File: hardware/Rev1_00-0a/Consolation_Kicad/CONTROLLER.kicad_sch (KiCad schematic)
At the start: 50 parts, among them J11 5051101092, J13 5051101092, J14 SFV5R-2STBE1HLF, J15 SFV5R-2STBE1HLF, U2 RP2350A, U7 ECS-2016MVQ-120-BP-TR, U8 GD25Q32CWIGR

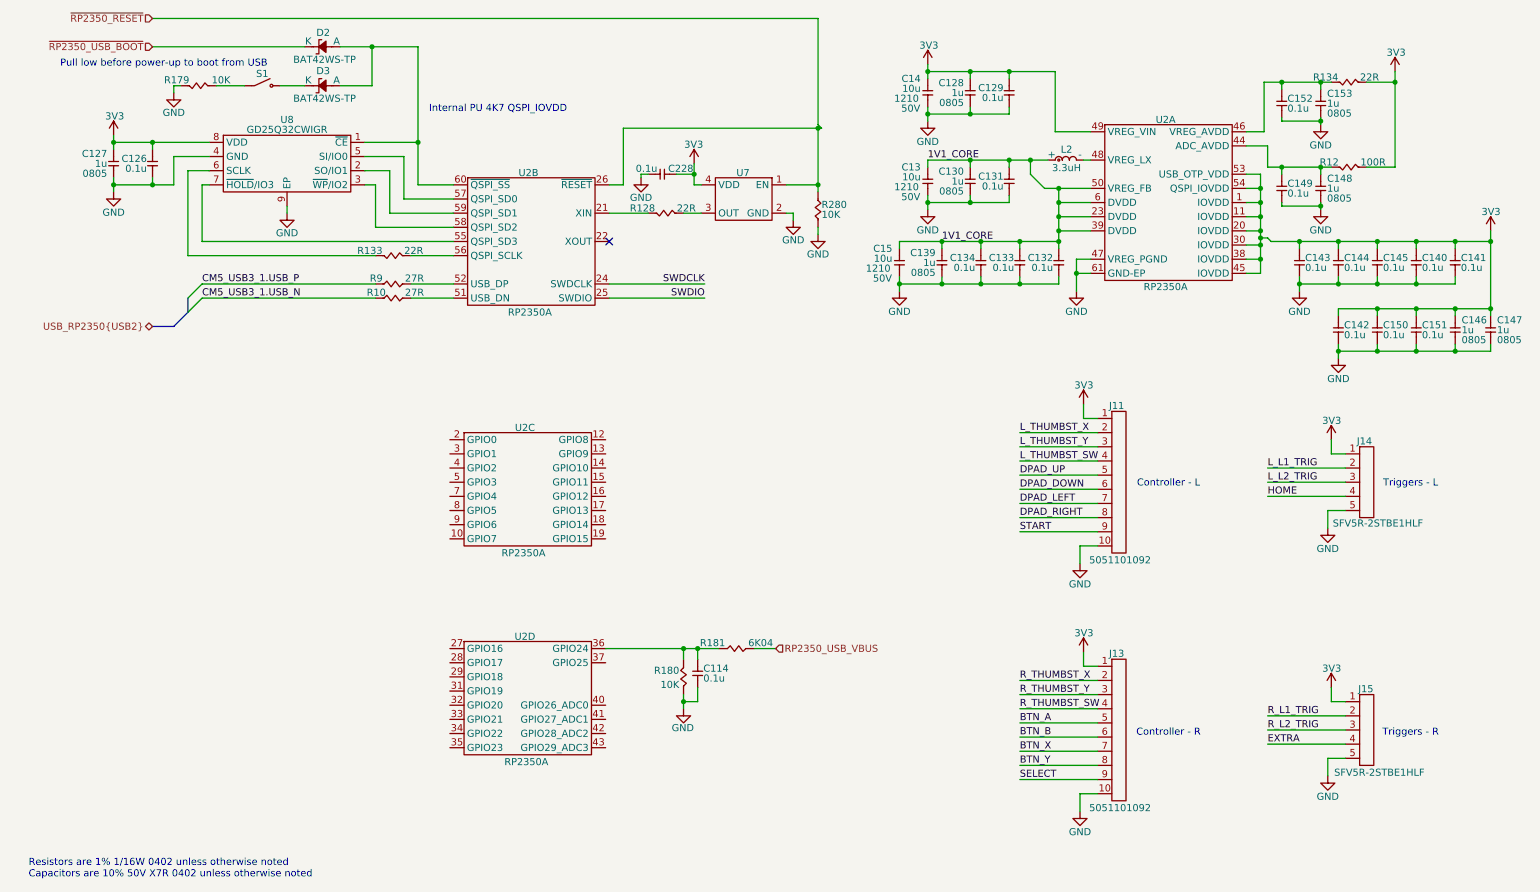
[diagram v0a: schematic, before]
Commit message: Update PinMux & Schematics
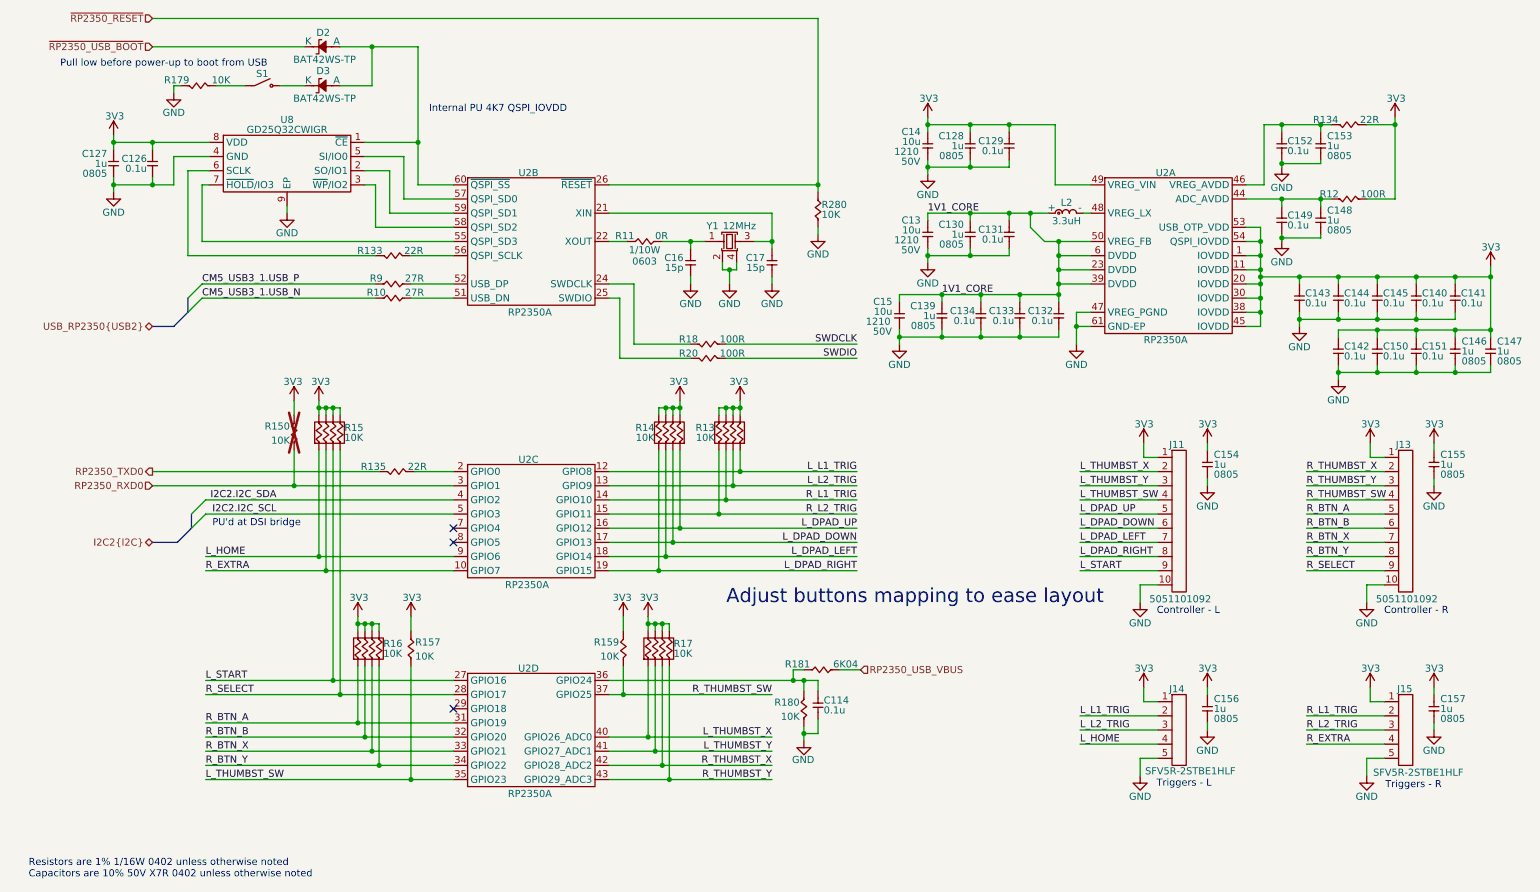
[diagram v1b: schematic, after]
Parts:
- removed C228: 0.1u, footprint:CAP_NONPOL_0402, symbol KicadCompDb:Capacitors/CAP_CER_SMT_00001
- removed R128: 22R, footprint:RES_0402, symbol KicadCompDb:Resistors/RES_SMT_00015
- removed U7: ECS-2016MVQ-120-BP-TR, footprint:4-SMD_2mmx1_6mm, symbol KicadCompDb:Oscillator/OSC_00003
- added C154, C155, C156, C157: 1u, footprint:CAP_NONPOL_0805, symbol KicadCompDb:Capacitors/CAP_CER_SMT_00002
- added C16, C17: 15p, footprint:CAP_NONPOL_0402, symbol KicadCompDb:Capacitors/CAP_CER_SMT_00019
- added R11: 0R, footprint:RES_0603, symbol KicadCompDb:Resistors/RES_SMT_00021
- added R13, R14, R15, R16, R17: 10K, footprint:RES_ARRAY_4_1206, symbol KicadCompDb:Resistors/RES_SMT_00037
- added R135: 22R, footprint:RES_0402, symbol KicadCompDb:Resistors/RES_SMT_00015
- added R150, R157, R159: 10K, footprint:RES_0402, symbol KicadCompDb:Resistors/RES_SMT_00013
- added R18, R20: 100R, footprint:RES_0402, symbol KicadCompDb:Resistors/RES_SMT_00035
- added Y1: 12MHz 10pF, footprint:4-SMD_3_2mmx2_5mm, symbol KicadCompDb:Crystals/CRYSTAL_00004
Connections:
- net BTN_A is gone; now on net R_BTN_A: J13.5
- net BTN_B is gone; now on net R_BTN_B: J13.6
- net BTN_X is gone; now on net R_BTN_X: J13.7
- net BTN_Y is gone; now on net R_BTN_Y: J13.8
- net DPAD_DOWN is gone; now on net L_DPAD_DOWN: J11.6
- net DPAD_LEFT is gone; now on net L_DPAD_LEFT: J11.7
- net DPAD_RIGHT is gone; now on net L_DPAD_RIGHT: J11.8
- net DPAD_UP is gone; now on net L_DPAD_UP: J11.5
- net EXTRA is gone; now on net R_EXTRA: J15.4
- net HOME is gone; now on net L_HOME: J14.4
- net SELECT is gone; now on net R_SELECT: J13.9
- net START is gone; now on net L_START: J11.9
- net 3V3: now also C154.2, C155.2, C156.2, C157.2, R13.5, R13.6, R13.7, R13.8, R14.5, R14.6, R14.7, R14.8, R15.5, R15.6, R15.7, R15.8, R150.2, R157.2, R159.2, R16.5, R16.6, R16.7, R16.8, R17.5, R17.6, R17.7, R17.8
- net GND: now also C154.1, C155.1, C156.1, C157.1, C16.1, C17.1, Y1.2 (GND), Y1.4 (GND)
- net L_L1_TRIG: now also U2.12 (GPIO8), R13.1
- net L_L2_TRIG: now also U2.13 (GPIO9), R13.2
- net L_THUMBST_SW: now also U2.35 (GPIO23), R157.1
- net L_THUMBST_X: now also U2.40 (GPIO26_ADC0), R17.1
- net L_THUMBST_Y: now also U2.41 (GPIO27_ADC1), R17.2
- net R_L1_TRIG: now also U2.14 (GPIO10), R13.3
- net R_L2_TRIG: now also U2.15 (GPIO11), R13.4
- net R_THUMBST_SW: now also U2.37 (GPIO25), R159.1
- net R_THUMBST_X: now also U2.42 (GPIO28_ADC2), R17.3
- net R_THUMBST_Y: now also U2.43 (GPIO29_ADC3), R17.4
- net SWDCLK: now also R18.1; no longer U2.24 (SWDCLK)
- net SWDIO: now also R20.1; no longer U2.25 (SWDIO)
- net at U2.21 (XIN): now also C17.2, Y1.3 (XO)
- net at U2.22 (XOUT): now also R11.1
- net R_EXTRA: now reaches U2.10 (GPIO7)
- net R_EXTRA: now also R15.2
- net L_DPAD_UP: now reaches U2.16 (GPIO12)
- net L_DPAD_UP: now also R14.1
- net L_DPAD_DOWN: now reaches U2.17 (GPIO13)
- net L_DPAD_DOWN: now also R14.2
- net L_DPAD_LEFT: now reaches U2.18 (GPIO14)
- net L_DPAD_LEFT: now also R14.3
- net L_DPAD_RIGHT: now reaches U2.19 (GPIO15)
- net L_DPAD_RIGHT: now also R14.4
- net at U2.2 (GPIO0): now also R135.1
- net RP2350_RXD0: now reaches U2.3 (GPIO1)
- net RP2350_RXD0: now also R150.1
- net I2C2.I2C_SDA: now reaches U2.4 (GPIO2)
- net I2C2.I2C_SCL: now reaches U2.5 (GPIO3)
- net L_HOME: now reaches U2.9 (GPIO6)
- net L_HOME: now also R15.1
- net L_START: now reaches U2.27 (GPIO16)
- net L_START: now also R15.3
- net R_SELECT: now reaches U2.28 (GPIO17)
- net R_SELECT: now also R15.4
- net R_BTN_A: now reaches U2.31 (GPIO19)
- net R_BTN_A: now also R16.1
- net R_BTN_B: now reaches U2.32 (GPIO20)
- net R_BTN_B: now also R16.2
- net R_BTN_X: now reaches U2.33 (GPIO21)
- net R_BTN_X: now also R16.3
- net R_BTN_Y: now reaches U2.34 (GPIO22)
- net R_BTN_Y: now also R16.4
- new net: R18.2, U2.24 (SWDCLK)
- new net: R20.2, U2.25 (SWDIO)
- new net: C16.2, R11.2, Y1.1 (XI)
- new net RP2350_TXD0: R135.2
- no-connect marks 1 -> 3
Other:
- note added: "Adjust buttons mapping to ease layout"
- note added: "PU'd at DSI bridge"
- moved on the sheet: C114, C128, C129, C13, C130, C131, C132, C133, C134, C139, C14, C140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
